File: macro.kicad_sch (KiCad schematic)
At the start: 62 parts, among them J1 Conn_01x01_Male, J2 Conn_01x01_Male, J3 Conn_01x01_Male, Q1 BSS138, SW1 RotaryEncoder_Switch, SW2 SW_Push, U1 AP2112K-3.3, U2 W25Q128JVPIQ, U3 RP2040, Y1 12MHz

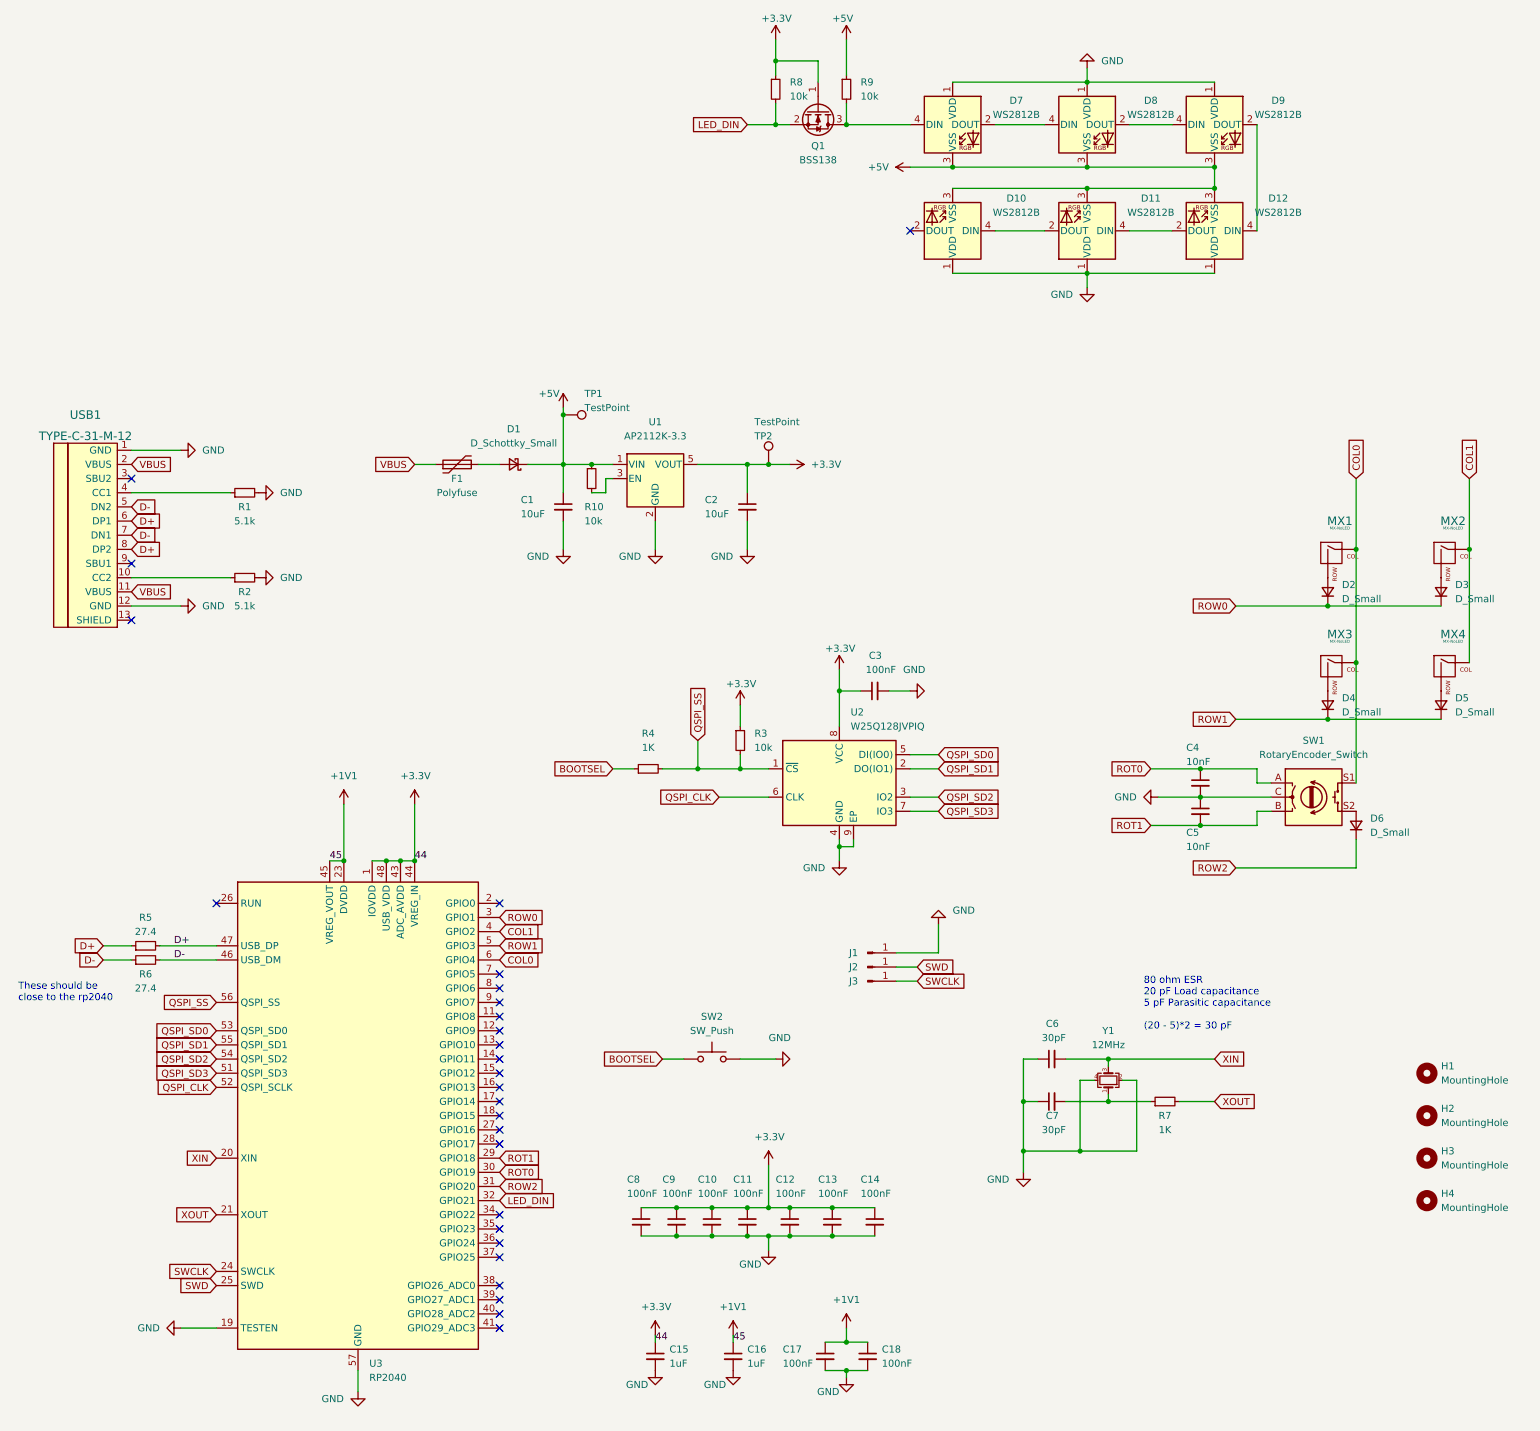
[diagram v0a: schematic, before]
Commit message: Cleanup schematic
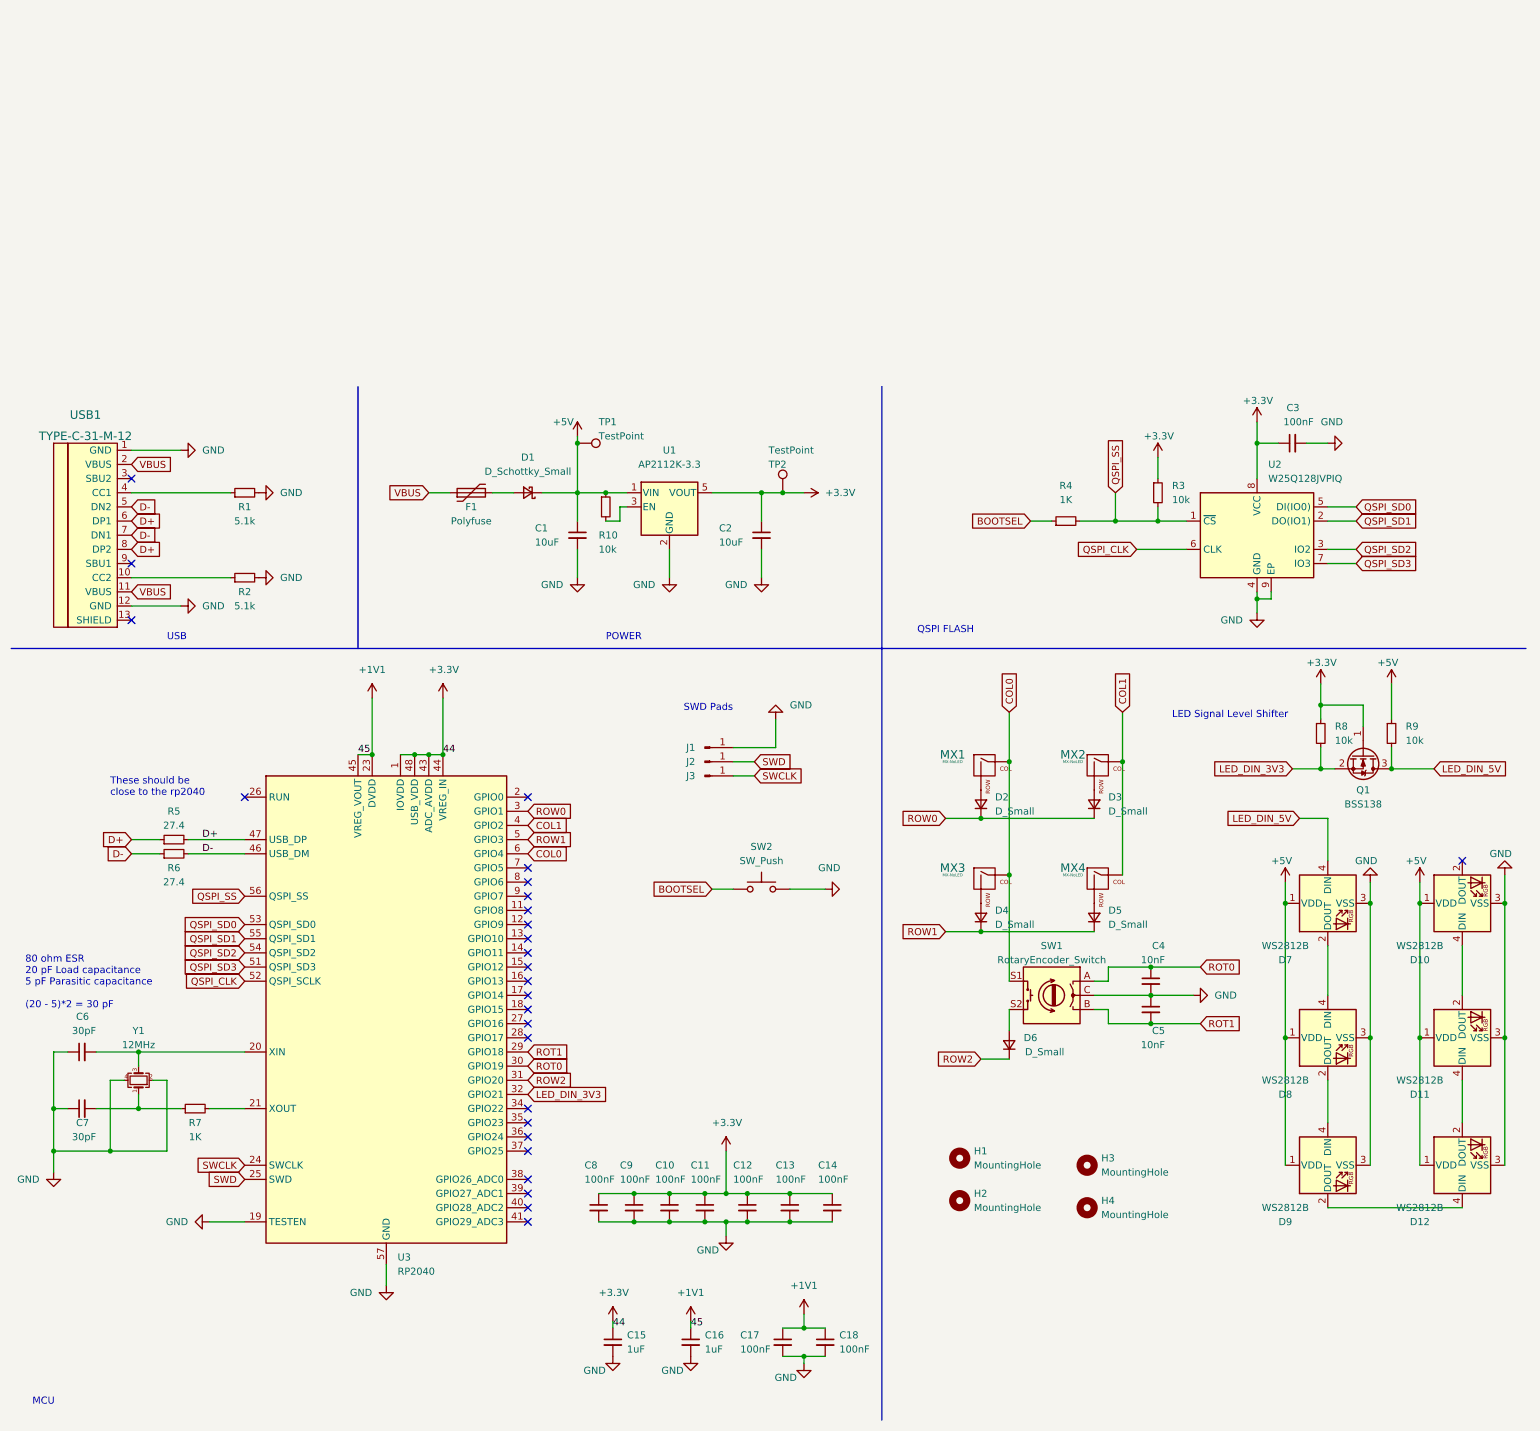
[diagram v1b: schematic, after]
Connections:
- net +5V: now also D10.1 (VDD), D11.1 (VDD), D12.1 (VDD), D7.1 (VDD), D8.1 (VDD), D9.1 (VDD); no longer D10.3 (VSS), D11.3 (VSS), D12.3 (VSS), D7.3 (VSS), D8.3 (VSS), D9.3 (VSS)
- net GND: now also D10.3 (VSS), D11.3 (VSS), D12.3 (VSS), D7.3 (VSS), D8.3 (VSS), D9.3 (VSS); no longer D10.1 (VDD), D11.1 (VDD), D12.1 (VDD), D7.1 (VDD), D8.1 (VDD), D9.1 (VDD)
- net LED_DIN_5V: now reaches D7.4 (DIN), Q1.3 (D), R9.2
- net LED_DIN renamed LED_DIN_3V3
- net XIN: no longer names the net of C6.2, U3.20 (XIN), Y1.3
- net XOUT: no longer names the net of R7.2, U3.21 (XOUT)
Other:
- note added: "LED Signal Level Shifter"
- note added: "MCU"
- note added: "POWER"
- note added: "QSPI FLASH"
- note added: "SWD Pads"
- note added: "USB"
- moved on the sheet: C1, C10, C11, C12, C13, C14, C15, C16, C17, C18, C2, C3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
